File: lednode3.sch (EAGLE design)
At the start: 40 parts, among them J1 POWER_JACKPTH, Q1 AO3402, Q2 AO3402, Q3 AO3402, Q4 AO3402, Q5 AO3402, Q6 AO3402

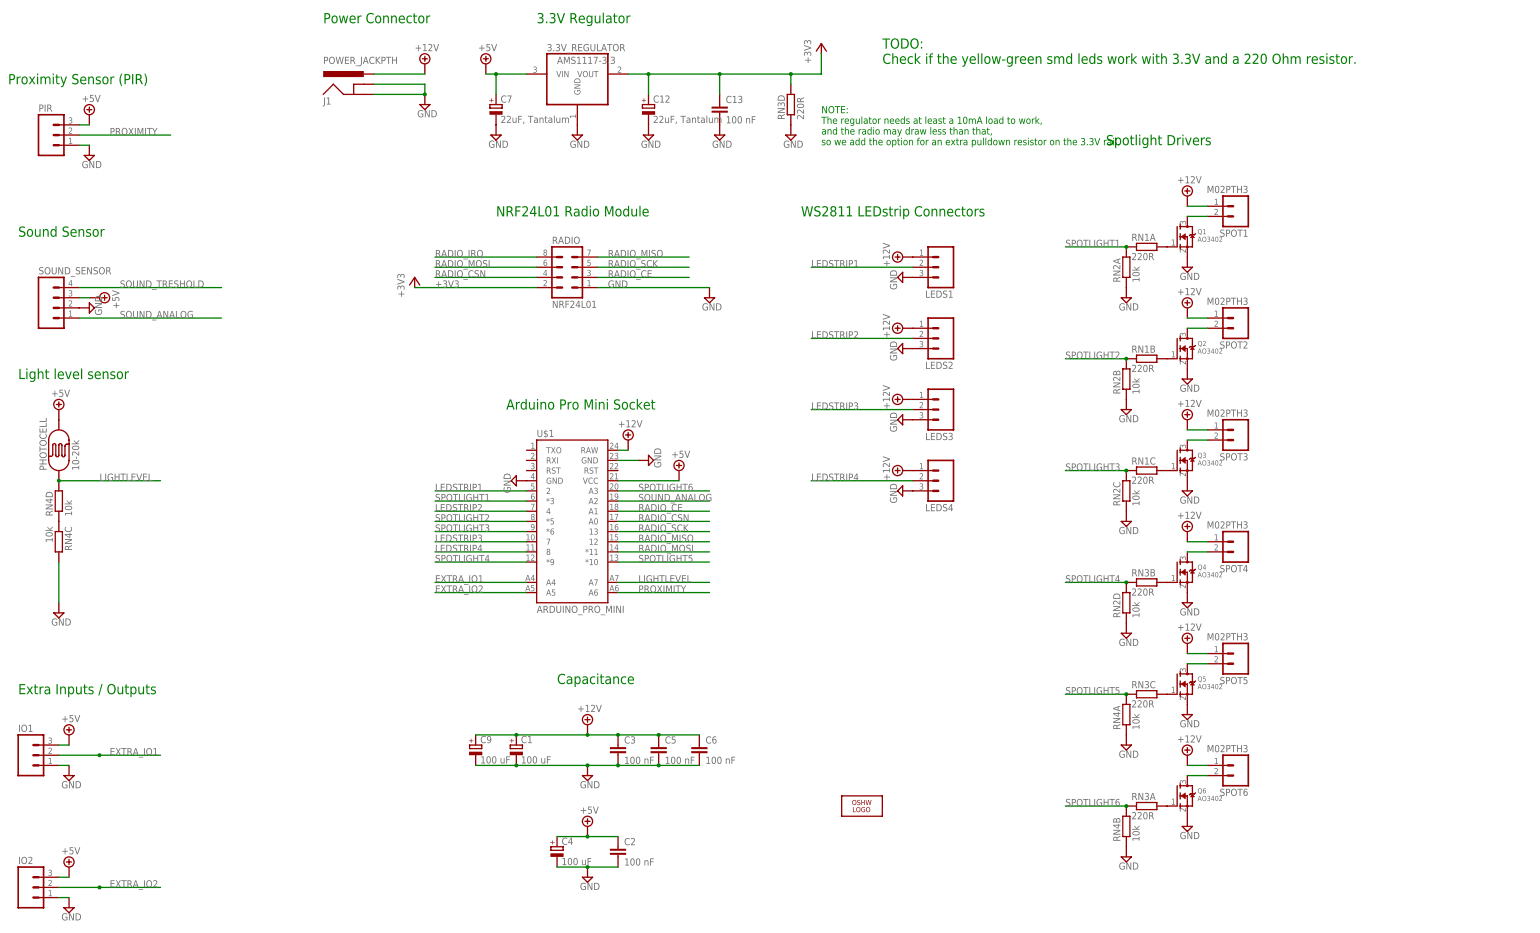
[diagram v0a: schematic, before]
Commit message: Finished lednode v 3.0.
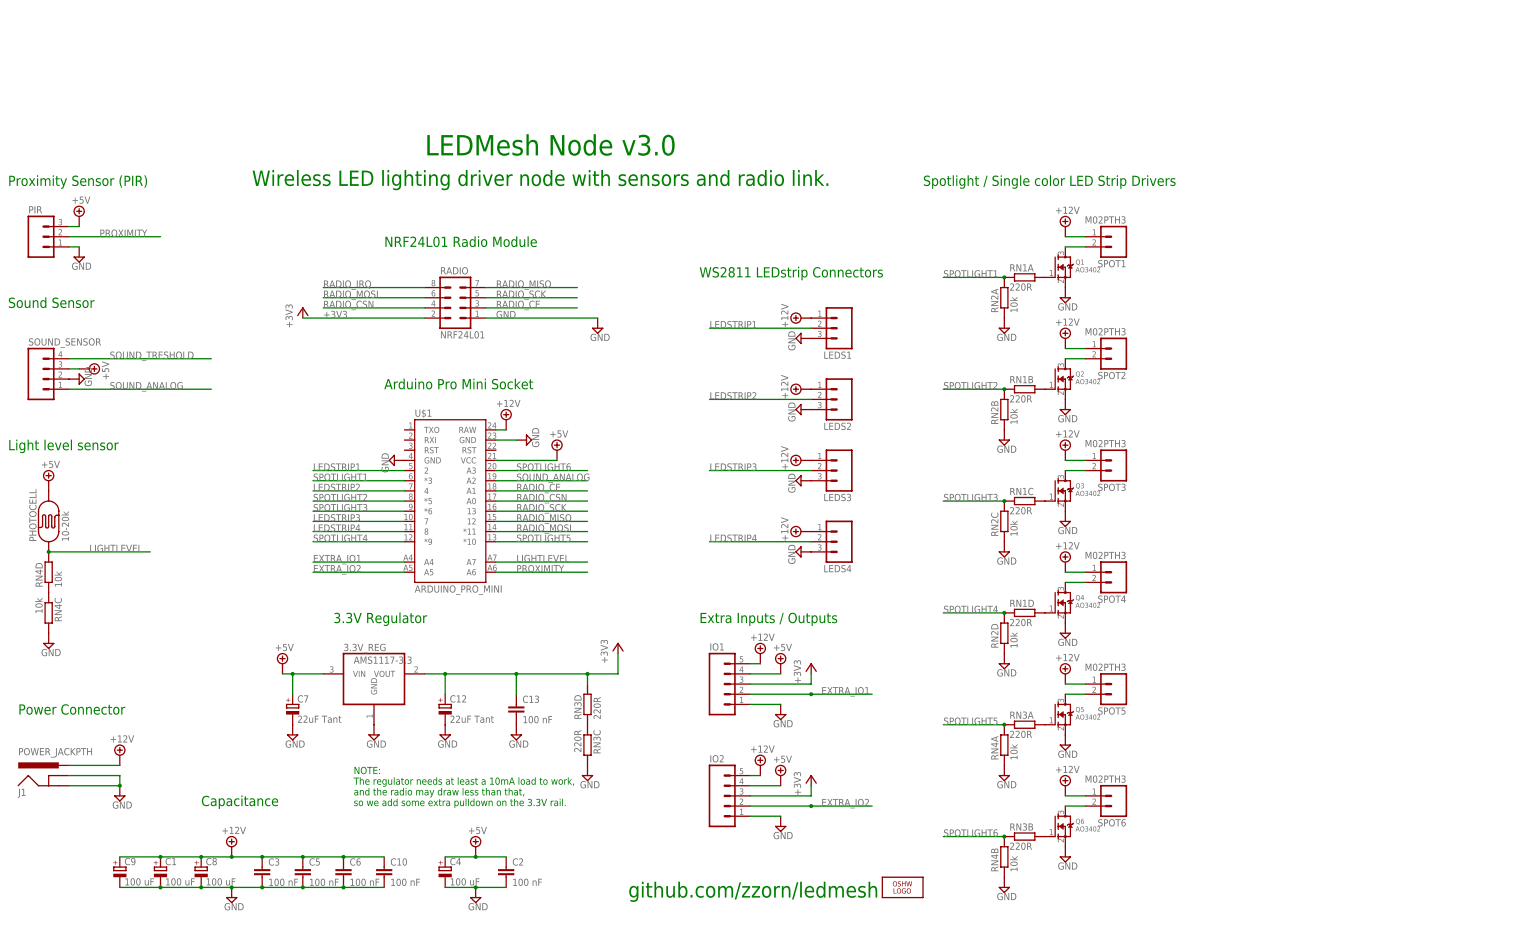
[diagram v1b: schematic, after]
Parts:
- removed 3.3V_REGULATOR: AMS1117-3.3, burr-brown:REG1117
- added 3.3V_REG: AMS1117-3.3, burr-brown:REG1117
- added C10: 100 nF, rcl:C-EUC0805
- added C8: 100 uF, rcl:CPOL-EUE2.5-6
- C12, C7: value 22uF, Tantalum -> 22uF Tant
- IO1, IO2: device SparkFun-Connectors:M03PTH -> SparkFun-Connectors:M05PTH
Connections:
- new net N$13: Q6.G, RN3B.2
- net +12V: now also C10.1, C8.+, IO1.5, IO2.5
- net +3V3: now also 3.3V_REG.VOUT, IO1.3, IO2.3; no longer 3.3V_REGULATOR.VOUT
- net +5V: now also 3.3V_REG.VIN, IO1.4, IO2.4; no longer 3.3V_REGULATOR.VIN, IO1.3, IO2.3
- net GND: now also 3.3V_REG.GND, C10.2, C8.-, RN3C.2; no longer 3.3V_REGULATOR.GND, RN3D.1
- net N$10: now also RN3A.2; no longer RN3C.2
- net N$14: now also RN3C.1, RN3D.1; no longer Q6.G, RN3A.2
- net N$8: now also RN1D.2; no longer RN3B.2
- net SPOTLIGHT4: now also RN1D.1; no longer RN3B.1
- net SPOTLIGHT5: now also RN3A.1; no longer RN3C.1
- net SPOTLIGHT6: now also RN3B.1; no longer RN3A.1
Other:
- note added: "LEDMesh Node v3.0"
- note added: "NOTE: The regulator needs at least a 10mA load to work, and the radio may draw less than that, so we add some extra pulldown on the 3.3V rail."
- note added: "Spotlight / Single color LED Strip Drivers"
- note added: "Wireless LED lighting driver node with sensors and radio link."
- note added: "github.com/zzorn/ledmesh"
- note removed: "NOTE: The regulator needs at least a 10mA load to work, and the radio may draw less than that, so we add the option for an extra pulldown resistor on the 3.3V rail."
- note removed: "Spotlight Drivers"
- note removed: "TODO: Check if the yellow-green smd leds work with 3.3V and a 220 Ohm resistor."
- moved on the sheet: C1, C12, C13, C2, C3, C4, C5, C6, C7, C9, J1, LEDS1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
